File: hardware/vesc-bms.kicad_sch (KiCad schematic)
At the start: 0 parts

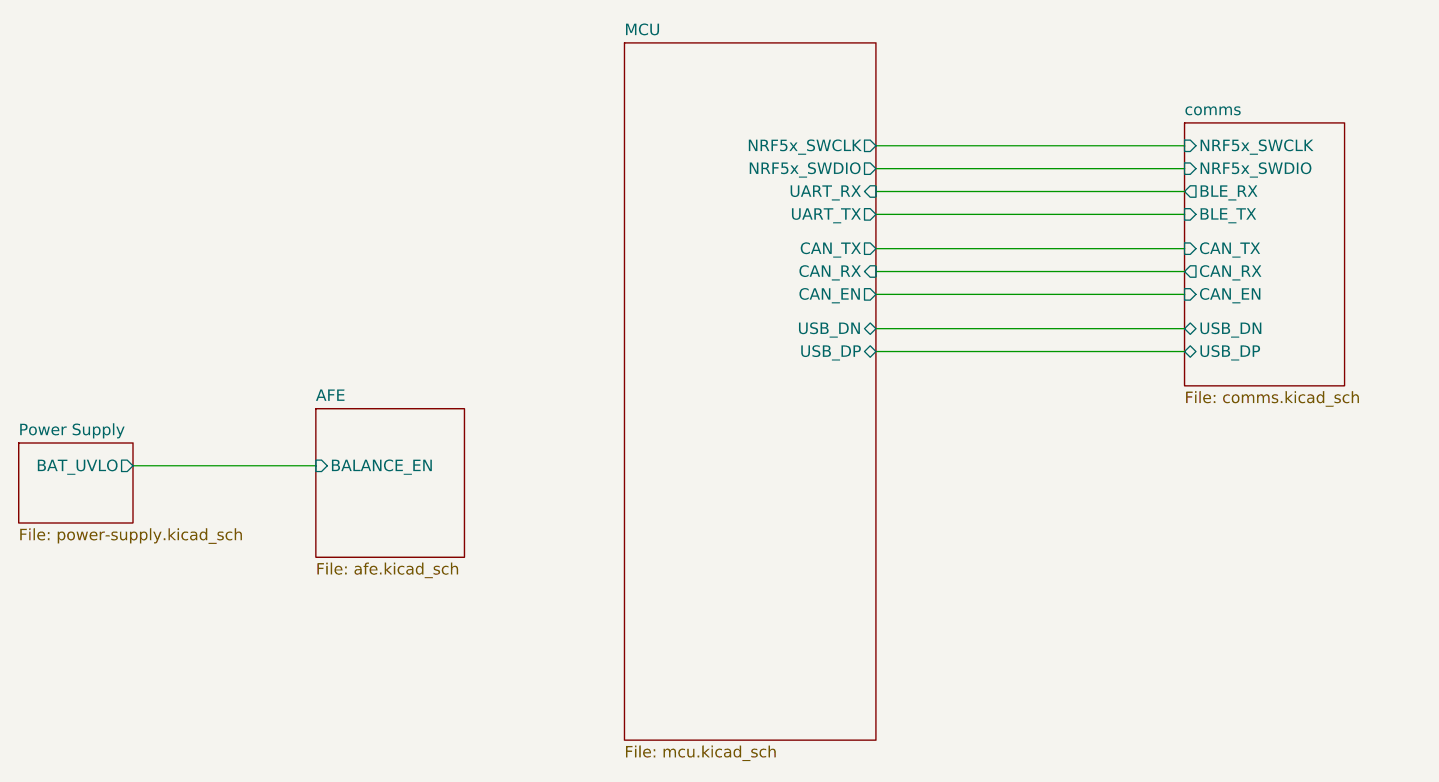
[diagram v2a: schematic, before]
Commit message: Analog front end ready
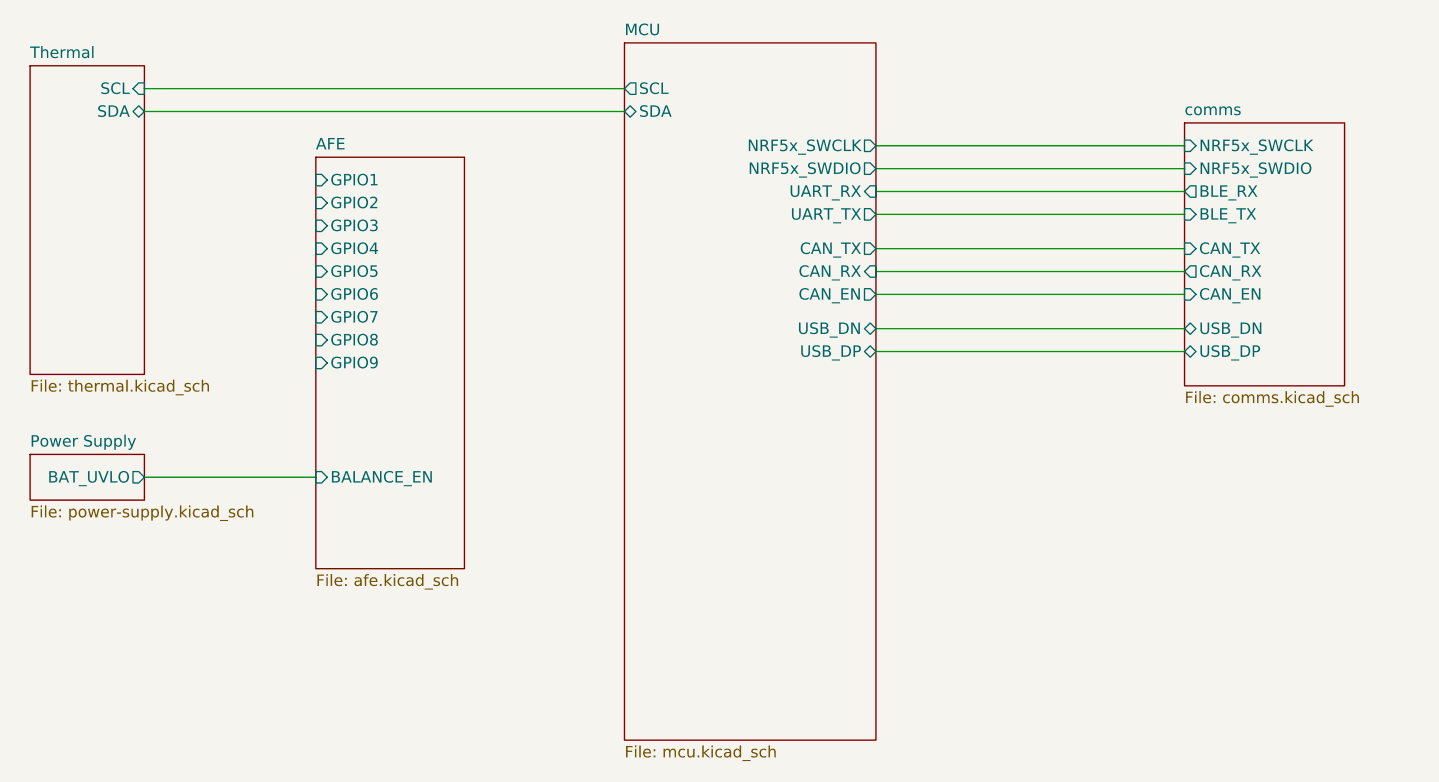
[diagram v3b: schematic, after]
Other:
- added sheet Thermal (thermal.kicad_sch)
- sheet AFE ports: added GPIO1, GPIO2, GPIO3, GPIO4, GPIO5, GPIO6, GPIO7, GPIO8, GPIO9; removed none
- sheet MCU ports: added SCL, SDA; removed none
